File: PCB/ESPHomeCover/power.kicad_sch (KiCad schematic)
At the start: 4 parts, among them X1 24V

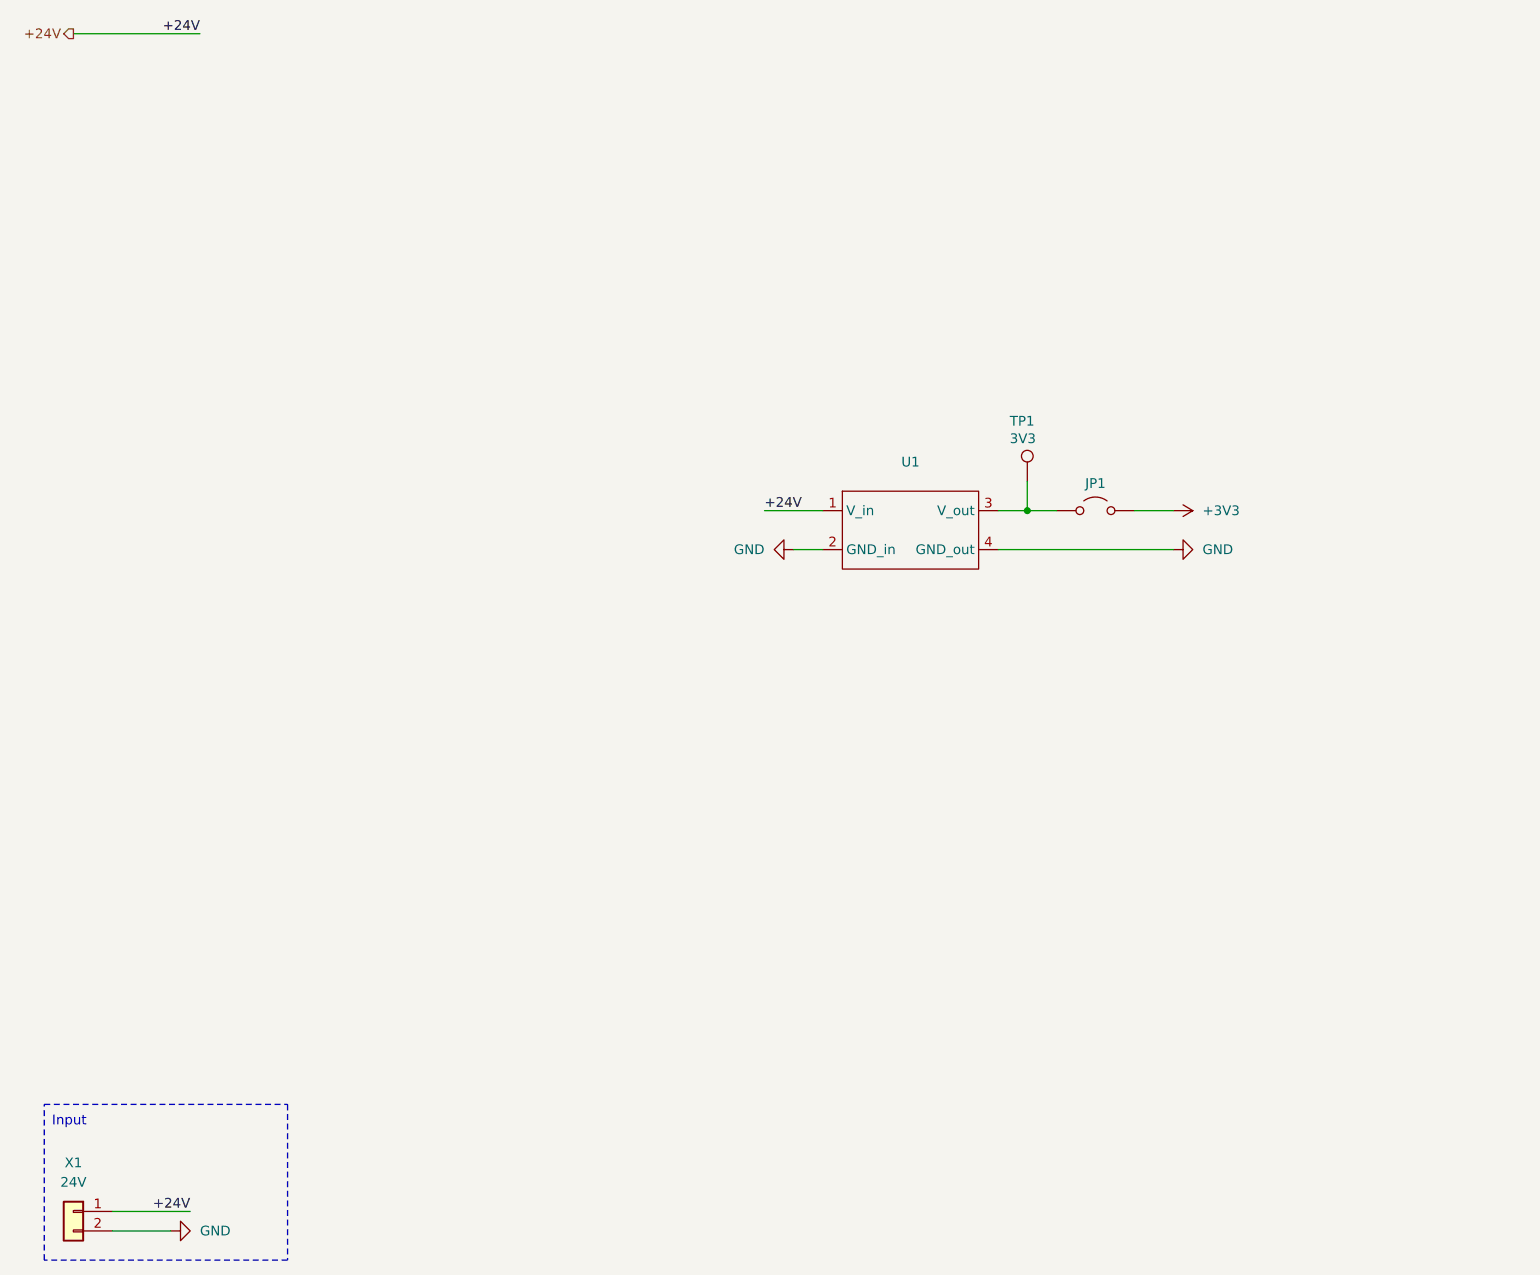
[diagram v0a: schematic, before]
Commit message: Add Board
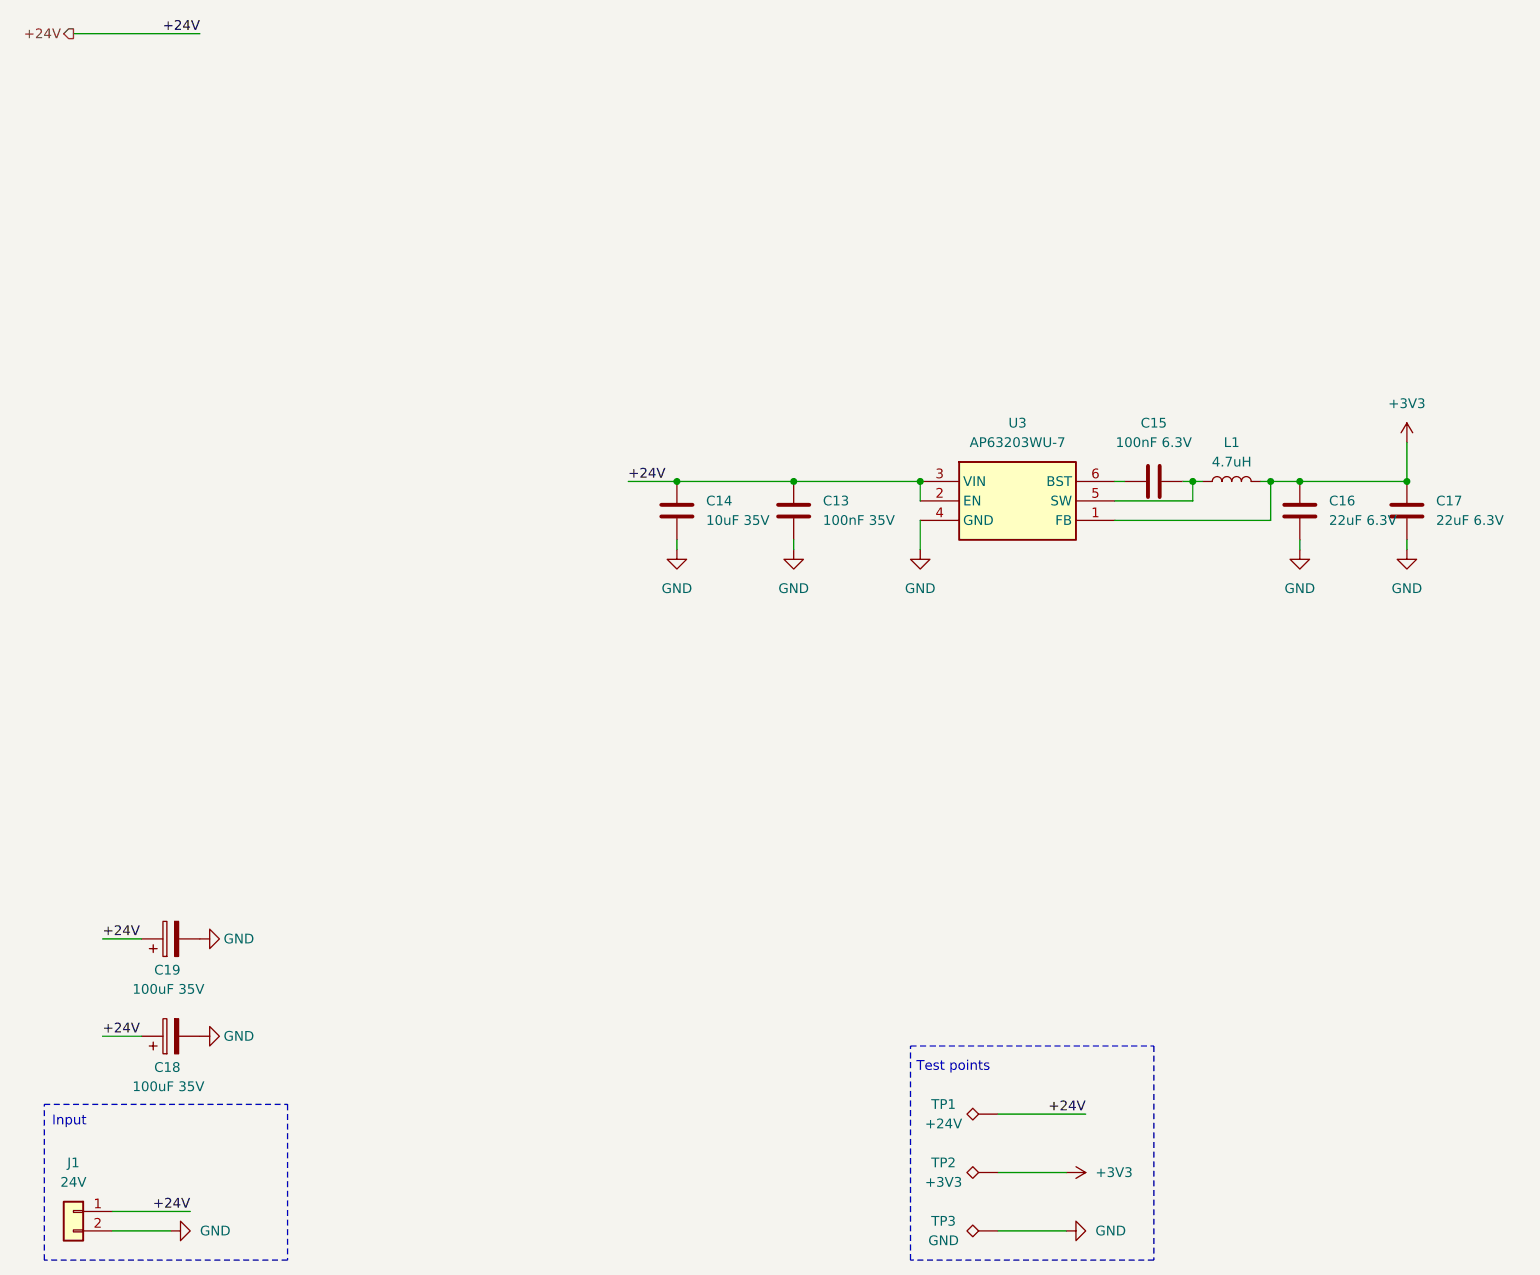
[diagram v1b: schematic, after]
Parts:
- removed JP1: ~, symbol Jumper:Jumper_2_Open
- removed TP1: 3V3, symbol Connector:TestPoint
- removed U1: ~, Own_Lib:LM2596S Modul, symbol own lib:LM2596S Modul
- added C13: 100nF 35V, Capacitor_SMD:C_0603_1608Metric, symbol Device:C
- added C14: 10uF 35V, Capacitor_SMD:C_0805_2012Metric, symbol Device:C
- added C15: 100nF 6.3V, Capacitor_SMD:C_0805_2012Metric, symbol Device:C
- added C16, C17: 22uF 6.3V, Capacitor_SMD:C_0805_2012Metric, symbol Device:C
- added C18, C19: 100uF 35V, Capacitor_SMD:CP_Elec_6.3x7.7, symbol Device:C_Polarized
- added L1: 4.7uH, Inductor_SMD:L_1812_4532Metric, symbol Device:L
- added TP1: +24V, TestPoint:TestPoint_Pad_2.0x2.0mm, symbol Connector:TestPoint_Alt
- added TP2: +3V3, TestPoint:TestPoint_Pad_2.0x2.0mm, symbol Connector:TestPoint_Alt
- added TP3: GND, TestPoint:TestPoint_Pad_2.0x2.0mm, symbol Connector:TestPoint_Alt
- added U3: AP63203WU-7, Package_TO_SOT_SMD:TSOT-23-6, symbol SamacSys_Parts:AP63203WU-7
- J1: renamed from X1; footprint (none) -> Connector_JST:JST_XH_B2B-XH-A_1x02_P2.50mm_Vertical
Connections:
- net +24V: now also C13.1, C14.1, C18.1, C19.1, TP1.1, U3.2 (EN), U3.3 (VIN)
- net +3V3: now also C16.1, C17.1, L1.2, TP2.1, U3.1 (FB)
- net GND: now also C13.2, C14.2, C16.2, C17.2, C18.2, C19.2, TP3.1, U3.4 (GND)
- new net: C15.1, U3.6 (BST)
- new net: C15.2, L1.1, U3.5 (SW)
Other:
- note added: "Test points"
